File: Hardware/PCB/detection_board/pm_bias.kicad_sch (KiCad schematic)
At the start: 21 parts, among them U1 MICROFC-60035-SMT-TR1, U2 LT1807, U3 ADCMP601

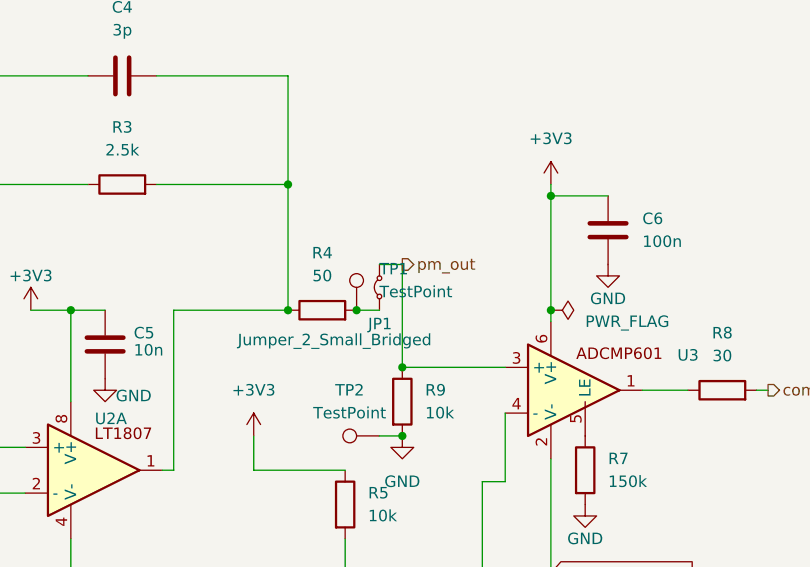
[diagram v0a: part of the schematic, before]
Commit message: nn
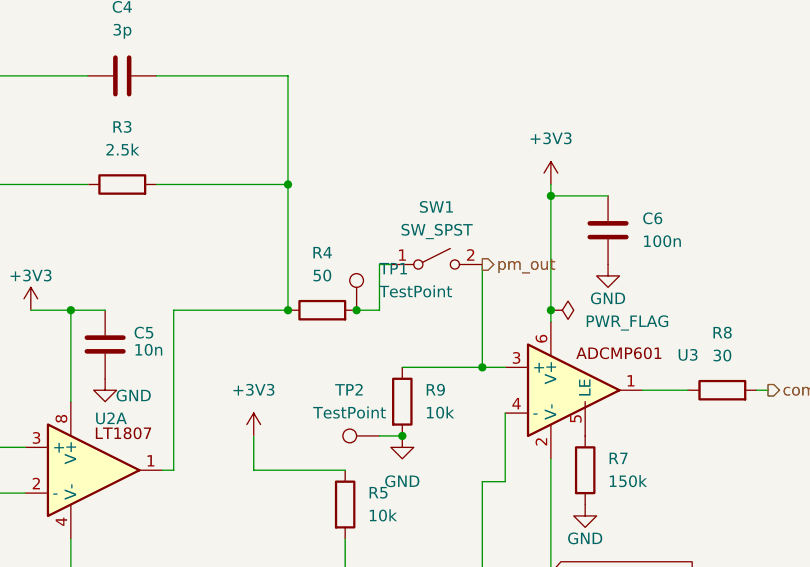
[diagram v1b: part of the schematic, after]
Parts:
- removed JP1: Jumper_2_Small_Bridged, TestPoint:TestPoint_2Pads_Pitch2.54mm_Drill0.8mm, symbol Jumper:Jumper_2_Small_Bridged
- added SW1: SW_SPST, Connector_PinHeader_2.54mm:PinHeader_1x03_P2.54mm_Vertical, symbol Switch:SW_SPST
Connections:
- net pm_out: now also SW1.2 (B)
- net at R4.2, TP1.1: now also SW1.1 (A)
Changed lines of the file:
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@@
 	)
 	(junction
-		(at 182.88 93.98)
+		(at 191.77 93.98)
 		(diameter 0)
 		(color 0 0 0 0)
@@
 	(wire
 		(pts
+			(xy 180.34 82.55) (xy 181.61 82.55)
+		)
+		(stroke
+			(width 0)
+			(type default)
+		)
+	)
+	(wire
+		(pts
 			(xy 146.05 113.03) (xy 146.05 118.11)
 		)
@@
 	(wire
 		(pts
-			(xy 182.88 82.55) (xy 182.88 93.98)
+			(xy 191.77 82.55) (xy 191.77 93.98)
 		)
 		(stroke
@@
 	(wire
 		(pts
+			(xy 180.34 87.63) (xy 180.34 82.55)
+		)
+		(stroke
+			(width 0)
+			(type default)
+		)
+	)
+	(wire
+		(pts
 			(xy 157.48 105.41) (xy 157.48 87.63)
 		)
@@
 	(wire
 		(pts
-			(xy 214.63 96.52) (xy 209.55 96.52)
+			(xy 182.88 93.98) (xy 194.31 93.98)
 		)
 		(stroke
@@
 	(wire
 		(pts
-			(xy 176.53 116.84) (xy 176.53 120.65)
+			(xy 214.63 96.52) (xy 209.55 96.52)
 		)
 		(stroke
@@
 	(wire
 		(pts
-			(xy 141.605 87.63) (xy 146.05 87.63)
+			(xy 176.53 116.84) (xy 176.53 120.65)
 		)
 		(stroke
@@
 	(wire
 		(pts
-			(xy 170.18 87.63) (xy 170.18 73.66)
+			(xy 141.605 87.63) (xy 146.05 87.63)
 		)
 		(stroke
@@
 	(wire
 		(pts
-			(xy 182.88 93.98) (xy 194.31 93.98)
+			(xy 170.18 87.63) (xy 170.18 73.66)
 		)
 		(stroke
@@
 		)
 	)
-	(wire
-		(pts
-			(xy 180.34 82.55) (xy 182.88 82.55)
-		)
-		(stroke
-			(width 0)
-			(type default)
-		)
-	)
 	(global_label "comparator_ret"
 		(shape input)
@@
 	(hierarchical_label "pm_out"
 		(shape output)
-		(at 182.88 82.55 0)
+		(at 191.77 82.55 0)
 		(effects
 			(font
@@
 	)
 	(symbol
-		(lib_id "Jumper:Jumper_2_Small_Bridged")
-		(at 180.34 85.09 90)
-		(unit 1)
-		(body_style 1)
-		(exclude_from_sim no)
-		(in_bom yes)
-		(on_board yes)
-		(in_pos_files yes)
-		(dnp no)
-		(property "Reference" "JP1"
-			(at 179.07 89.154 90)
-			(show_name no)
-			(do_not_autoplace no)
-			(effects
-				(font
-					(size 1.27 1.27)
-				)
-				(justify right)
-			)
-		)
-		(property "Value" "Jumper_2_Small_Bridged"
-			(at 164.592 90.932 90)
-			(show_name no)
-			(do_not_autoplace no)
-			(effects
-				(font
-					(size 1.27 1.27)
-				)
-				(justify right)
-			)
-		)
-		(property "Footprint" "TestPoint:TestPoint_2Pads_Pitch2.54mm_Drill0.8mm"
-			(at 180.34 85.09 0)
-			(hide yes)
-			(show_name no)
-			(do_not_autoplace no)
-			(effects
-				(font
-					(size 1.27 1.27)
-				)
-			)
-		)
-		(property "Datasheet" ""
-			(at 180.34 85.09 0)
-			(hide yes)
-			(show_name no)
-			(do_not_autoplace no)
-			(effects
-				(font
-					(size 1.27 1.27)
-				)
-			)
-		)
-		(property "Description" "Jumper, 2-pole, small symbol, bridged"
-			(at 180.34 85.09 0)
-			(hide yes)
-			(show_name no)
-			(do_not_autoplace no)
-			(effects
-				(font
-					(size 1.27 1.27)
-				)
-			)
-		)
-		(pin "2"
-		)
-		(pin "1"
-		)
-		(instances
-			(project "detection_board"
-				(path "/871ea243-9d20-4c93-850f-9fe294f22536/08fd595b-02df-4a61-8399-858a89ae5419"
-					(reference "JP1")
-					(unit 1)
-				)
-			)
-		)
-	)
-	(symbol
 		(lib_id "power:GND")
 		(at 146.05 118.11 0)
@@
 					(unit 1)
 				)
+			)
+		)
+	)
+	(symbol
+		(lib_id "Switch:SW_SPST")
+		(at 186.69 82.55 0)
+		(unit 1)
+		(body_style 1)
+		(exclude_from_sim no)
+		(in_bom yes)
+		(on_board yes)
+		(in_pos_files yes)
+		(dnp no)
+		(fields_autoplaced yes)
+		(property "Reference" "SW1"
+			(at 186.69 76.2 0)
+			(show_name no)
+			(do_not_autoplace no)
+			(effects
+				(font
+					(size 1.27 1.27)
+				)
+			)
+		)
+		(property "Value" "SW_SPST"
+			(at 186.69 78.74 0)
+			(show_name no)
+			(do_not_autoplace no)
+			(effects
+				(font
+					(size 1.27 1.27)
+				)
+			)
+		)
+		(property "Footprint" "Connector_PinHeader_2.54mm:PinHeader_1x03_P2.54mm_Vertical"
+			(at 186.69 82.55 0)
+			(hide yes)
+			(show_name no)
+			(do_not_autoplace no)
+			(effects
+				(font
+					(size 1.27 1.27)
+				)
+			)
+		)
+		(property "Datasheet" ""
+			(at 186.69 82.55 0)
+			(hide yes)
+			(show_name no)
+			(do_not_autoplace no)
+			(effects
+				(font
+					(size 1.27 1.27)
+				)
+			)
+		)
+		(property "Description" "Single Pole Single Throw (SPST) switch"
+			(at 186.69 82.55 0)
+			(hide yes)
+			(show_name no)
+			(do_not_autoplace no)
+			(effects
+				(font
+					(size 1.27 1.27)
+				)
+			)
+		)
+		(pin "2"
+		)
+		(pin "1"
+		)
+		(instances
+			(project "detection_board"
+				(path "/871ea243-9d20-4c93-850f-9fe294f22536/08fd595b-02df-4a61-8399-858a89ae5419"
+					(reference "SW1")
+					(unit 1)
+				)
